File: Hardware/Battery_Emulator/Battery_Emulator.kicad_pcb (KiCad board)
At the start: 2 copper layers, 33 x 89.1 mm, 50 parts, among them J1 Vin, J2 USB4105-GF-A-060, J3 Cell1_Vout, Q1 IRFB7545PBF, SW1 Jumper, SW2 Jumper, U1 MCP4651T-103E_ST, U10 ATmega328PB-A, U2 ISO1640BDR, U3 74AHC2G125DP,125, U4 FT230XS-R, U5 LM7805_TO220, U6 LM7805_TO220, U7 LM317_TO-220, U8 MCP6001UT-I/OT, Y1 Crystal_GND24

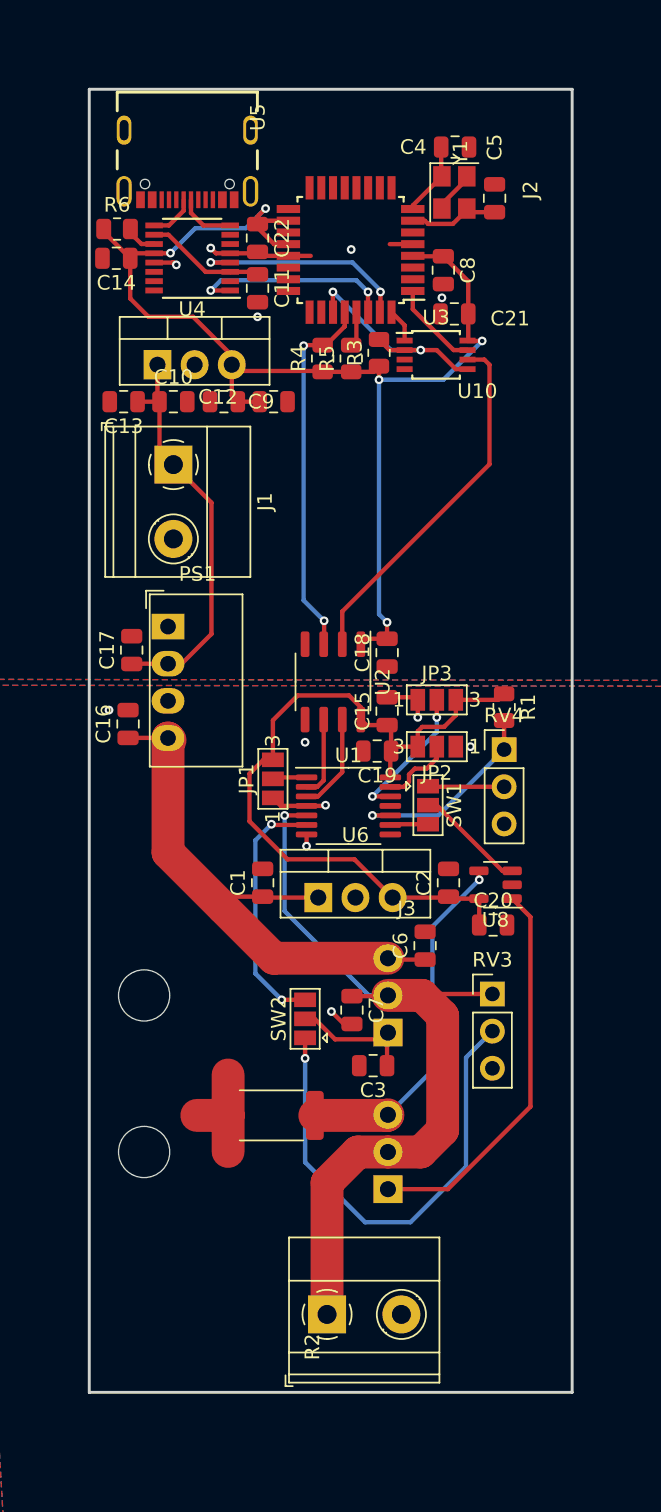
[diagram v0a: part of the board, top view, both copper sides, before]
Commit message: Update PCB design
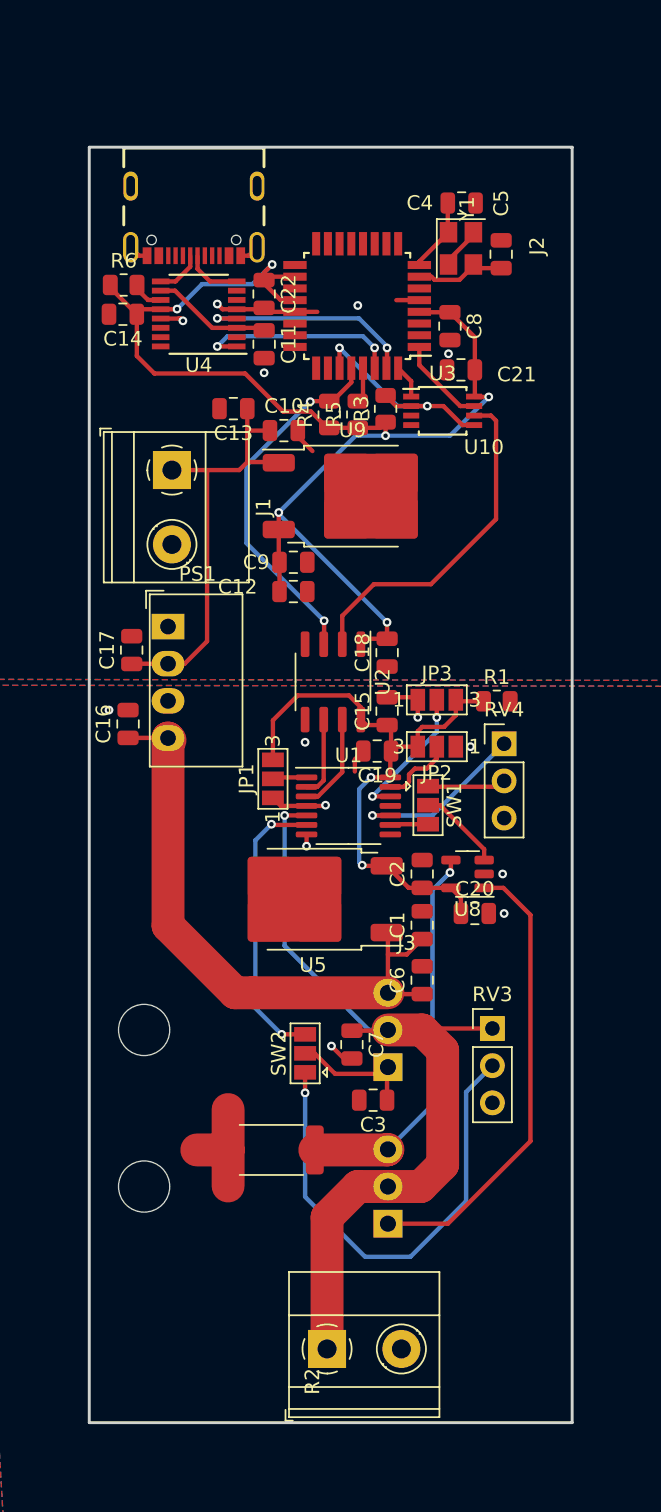
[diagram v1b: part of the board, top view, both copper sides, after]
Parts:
- removed U6: LM7805_TO220, Package_TO_SOT_THT:TO-220-3_Vertical
- added U9: KA78M05_TO252, Package_TO_SOT_SMD:TO-252-2, F.Cu at (59.8, 76.8)
- U5: value LM7805_TO220 -> KA78M05_TO252; footprint Package_TO_SOT_THT:TO-220-3_Vertical -> Package_TO_SOT_SMD:TO-252-2
- moved U5 38.0 mm to (57.1, 104.3), turned to 180 degrees
- moved C12 13.0 mm to (55.8, 83.3)
- moved C9 12.0 mm to (55.8, 81.3), turned to 0 degrees
- moved C1 11.3 mm to (64.6, 106.1)
- moved C10 7.80 mm to (55.1, 72.3)
- moved C13 7.52 mm to (51.7, 70.8)
- moved C21 3.85 mm to (67.2, 68.2)
- moved C22 3.85 mm to (53.8, 63.0)
- moved C4 3.85 mm to (67.3, 56.8)
- moved C5 3.85 mm to (70.0, 60.2)
- moved C8 3.85 mm to (66.5, 65.2)
- moved R3 3.85 mm to (62.1, 70.8)
- moved R4 3.85 mm to (58.2, 71.2)
- moved R5 3.85 mm to (60.2, 71.2)
- moved R6 3.85 mm to (44.2, 62.4)
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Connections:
- U5 pad 1: +12V -> /Cell_1/+9V_ISO
- U5 pad 2: GND -> /Cell_1/GND_ISO
- U5 pad 3: +5V -> /Cell_1/+5V_ISO
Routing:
- net /Cell_1/+5V_ISO: track 51.9 -> 41.8 mm, vias 0 -> 2
- net Net-(Q1-Pad1): track 26.8 -> 31.5 mm
- net GND: track 13.2 -> 17.7 mm
- net +5V: track 84.9 -> 89.0 mm, vias 5 -> 6
- net /Cell_1/+9V_ISO: track 38.2 -> 42.0 mm
- net +12V: track 27.7 -> 30.2 mm
- net /Cell_1/COUT+: track 55.5 -> 57.8 mm
- net Net-(SW2-C): track 17.2 -> 19.6 mm
- net Net-(U8A--): track 24.3 -> 26.6 mm
- net Net-(U1-P0B): track 14.1 -> 12.3 mm
- net /Cell_1/GND_ISO: track 17.1 -> 18.8 mm, vias 7 -> 9
- net /SDA_cell_1-7: track 24.9 -> 23.6 mm
- net Net-(SW1-B): track 7.61 -> 6.42 mm
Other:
- board size 33 x 89.1 mm -> 33 x 87.2 mm
